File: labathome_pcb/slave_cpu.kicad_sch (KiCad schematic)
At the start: 29 parts, among them J26 EXT, J27 ADDA, J36 PROG_STM, U16 LM358, U5 STM32G431R8Tx

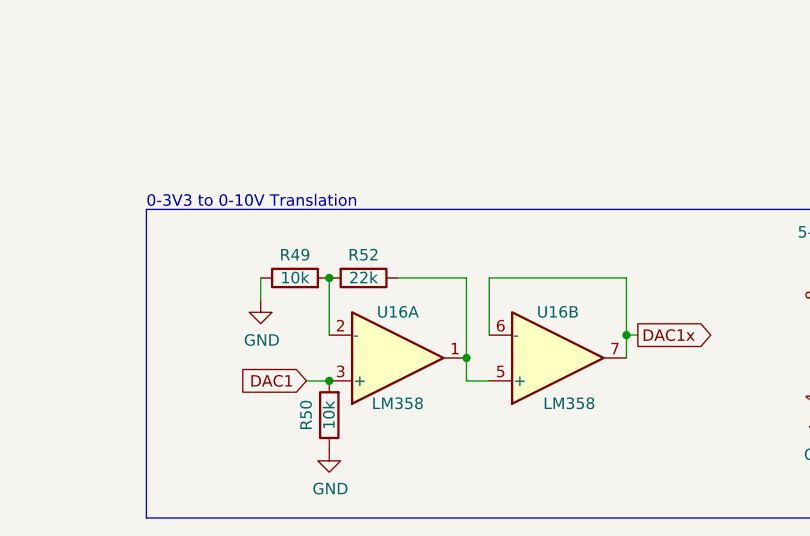
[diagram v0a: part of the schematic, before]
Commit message: Lab@Home 15.3 PCB as ordered @ JLCPCB
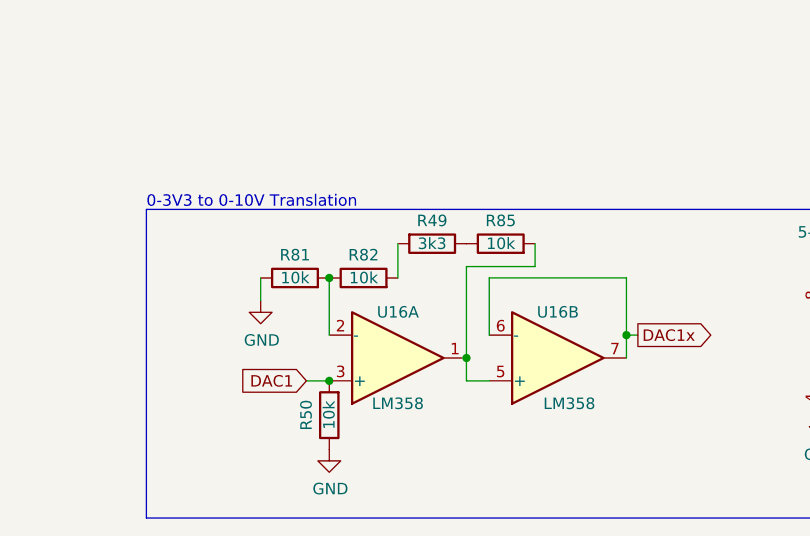
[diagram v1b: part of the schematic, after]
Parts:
- removed R52: 22k, Resistor_SMD:R_0805_2012Metric_Pad1.20x1.40mm_HandSolder, symbol Device:R
- added R81, R82, R85: 10k, Resistor_SMD:R_0201_0603Metric, symbol Device:R
- R49: value 10k -> 3k3; footprint Resistor_SMD:R_0805_2012Metric_Pad1.20x1.40mm_HandSolder -> Resistor_SMD:R_0402_1005Metric; MPN (none) -> 0402WGF3301TCE; Manufacturer (none) -> UNI-ROYAL(Uniroyal Elec)
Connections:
- net GND: now also R81.1; no longer R49.1
- net at U16.1, U16.5 (+): now also R85.2
- net at U16.2 (-): now also R81.2, R82.1; no longer R49.2
- new net: R49.1, R85.1
- new net: R49.2, R82.2
